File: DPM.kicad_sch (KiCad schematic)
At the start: 17 parts, among them J1 Conn_01x08, U1 74HC590, U2 74HC682, U3 ADG333A, U4 MCP23017_SP, U5 ADG333A

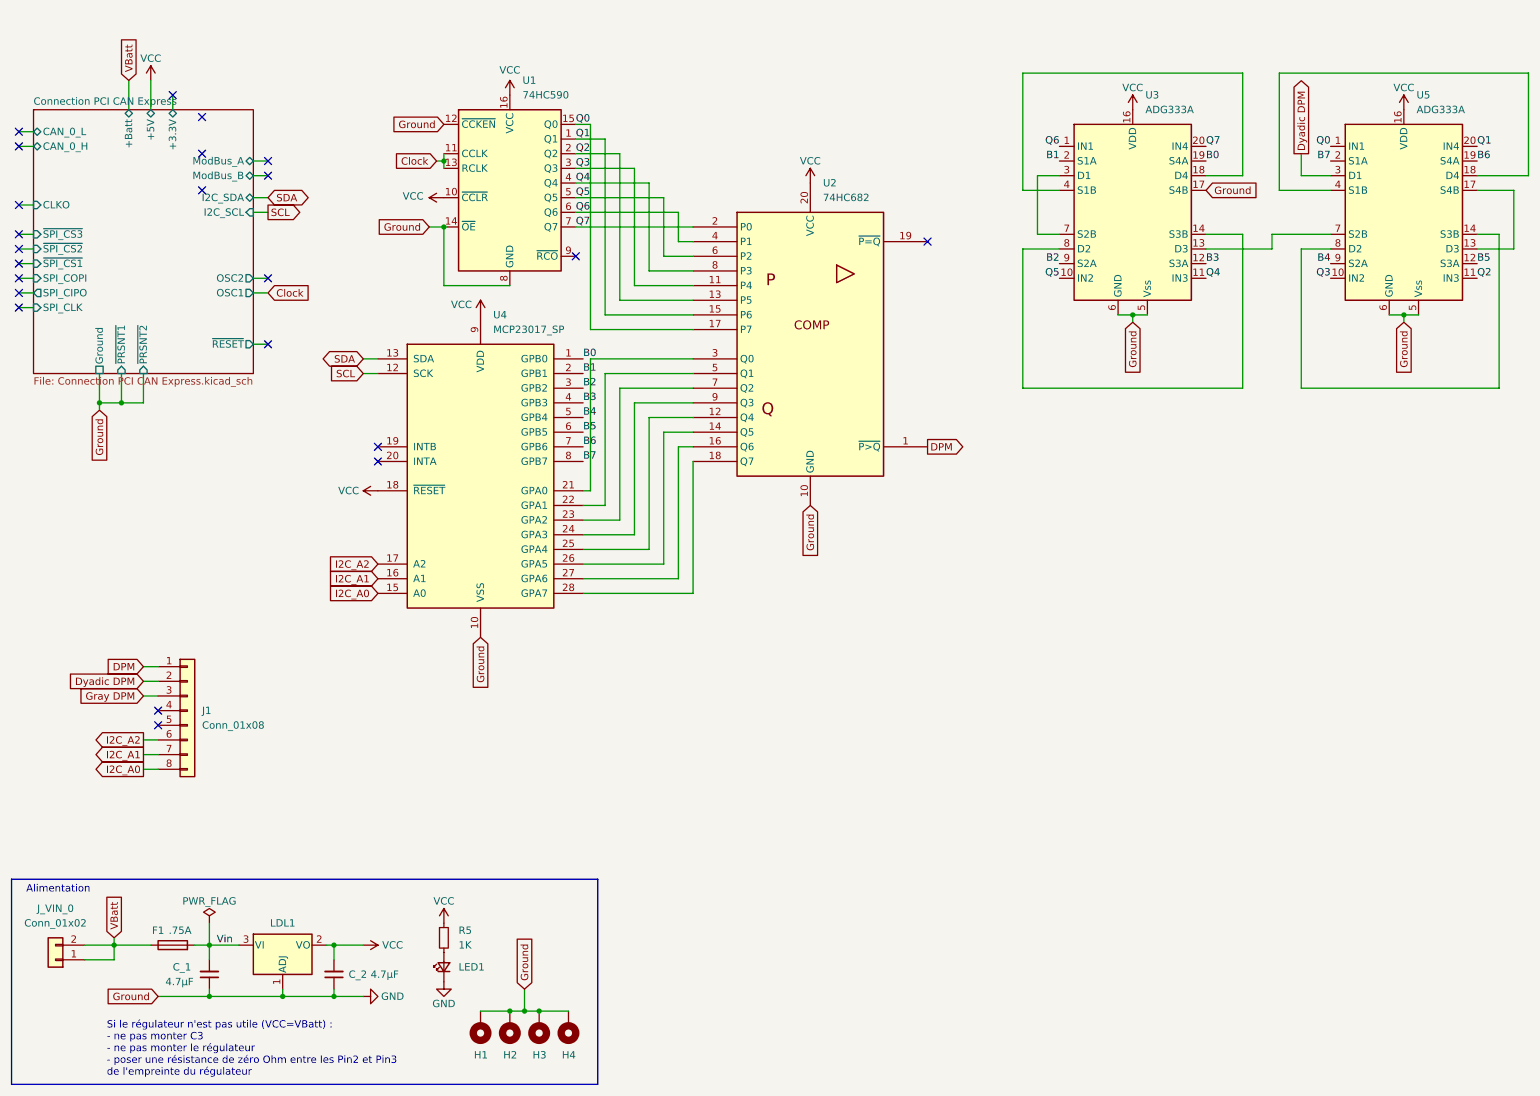
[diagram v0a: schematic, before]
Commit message: + 3 fonctionnalités : PWM, DPM & DDPM + début du routage de la carte
git-svn-id: file:///D%5C00%20-%20Dev%20&%20Calculs%5CRepoTortoiseSVN_PCB%5CD-DPM/trunk@16 f29d8339-a183-0348-962e-9e4594cf8312
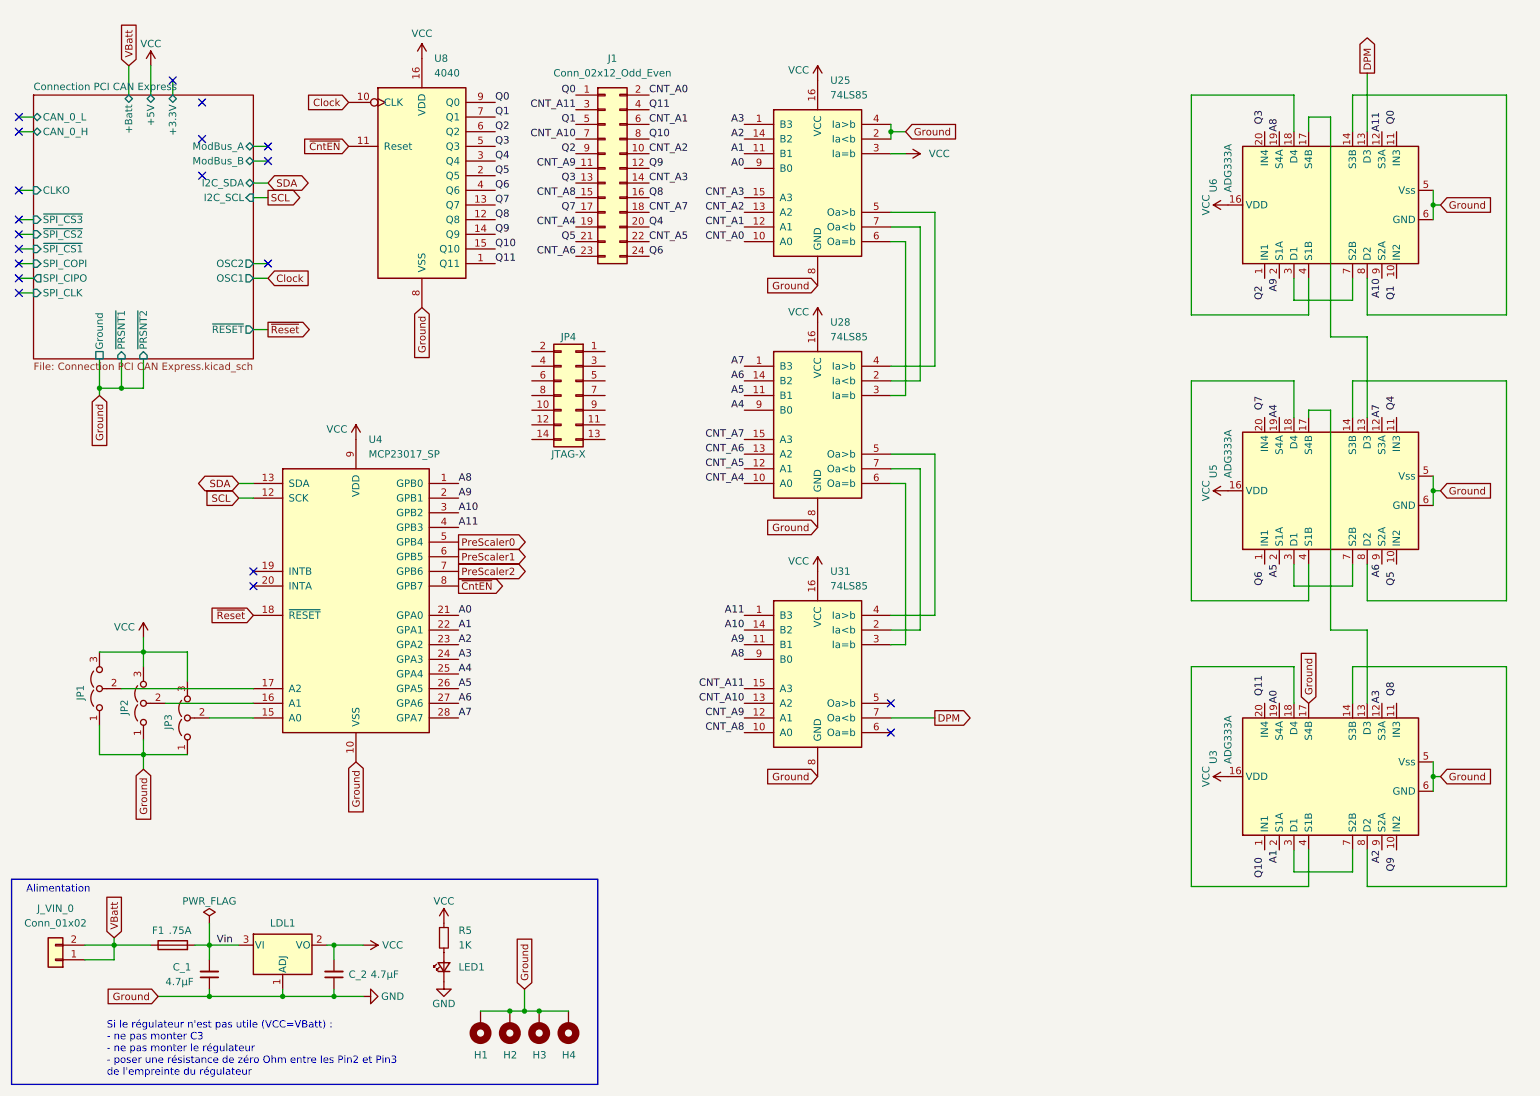
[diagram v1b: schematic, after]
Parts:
- removed J1: Conn_01x08, Connector_PinHeader_2.54mm:PinHeader_1x08_P2.54mm_Vertical, symbol Connector_Generic:Conn_01x08
- removed U1: 74HC590, Package_DIP:DIP-16_W7.62mm_Socket_LongPads, symbol Perso_Spare_parts:74HC590
- removed U2: 74HC682, Package_DIP:DIP-20_W7.62mm_Socket_LongPads, symbol Perso_Spare_parts:74HC682
- added J1: Conn_02x12_Odd_Even, Connector_PinHeader_2.54mm:PinHeader_2x12_P2.54mm_Vertical, symbol Connector_Generic:Conn_02x12_Odd_Even
- added JP1, JP2, JP3: Jumper_3_Open, Connector_PinHeader_2.54mm:PinHeader_1x03_P2.54mm_Vertical, symbol Jumper:Jumper_3_Open
- added JP4: JTAG-X, Connector_IDC:IDC-Header_2x07_P2.54mm_Horizontal, symbol Connector_Generic:Conn_02x07_Odd_Even
- added U25, U28, U31: 74LS85, Package_DIP:DIP-16_W7.62mm_Socket, symbol 74xx:74LS85
- added U6: ADG333A, Package_DIP:DIP-20_W7.62mm_Socket_LongPads, symbol Perso_Spare_parts:ADG333A
- added U8: 4040, Package_DIP:DIP-16_W7.62mm_Socket, symbol 4xxx:4040
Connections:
- net Clock: now also U8.10 (CLK)
- net DPM: now also U31.7 (Oa<b), U6.13 (D3)
- net GND: now also JP1.1 (A), JP2.1 (A), JP3.1 (A), U25.2 (Ia<b), U25.4 (Ia>b), U25.8 (GND), U28.8 (GND), U31.8 (GND), U6.15 (NC), U6.5 (Vss), U6.6 (GND), U8.8 (VSS)
- net Q0: now also J1.1 (Pin_1), U8.9 (Q0); no longer U5.1 (IN1)
- net Q1: now also J1.5 (Pin_5), U8.7 (Q1); no longer U5.20 (IN4)
- net Q2: now also J1.9 (Pin_9), U8.6 (Q2); no longer U5.11 (IN3)
- net Q3: now also J1.13 (Pin_13), U8.5 (Q3); no longer U5.10 (IN2)
- net Q4: now also J1.20 (Pin_20), U8.3 (Q4); no longer U3.11 (IN3)
- net Q5: now also J1.21 (Pin_21), U8.2 (Q5); no longer U3.10 (IN2)
- net Q6: now also J1.24 (Pin_24), U8.4 (Q6); no longer U3.1 (IN1)
- net Q7: now also J1.17 (Pin_17), U8.13 (Q7); no longer U3.20 (IN4)
- net VCC: now also JP1.3 (B), JP2.3 (B), JP3.3 (B), U25.16 (VCC), U25.3 (Ia=b), U28.16 (VCC), U31.16 (VCC), U6.16 (VDD), U8.16 (VDD); no longer U4.18 (~{RESET})
- net A0: now reaches U4.21 (GPA0)
- net A0: now also U3.19 (S4A), U25.9 (B0)
- net A1: now reaches U4.22 (GPA1)
- net A1: now also U3.2 (S1A), U25.11 (B1)
- net A2: now reaches U4.23 (GPA2)
- net A2: now also U3.9 (S2A), U25.14 (B2)
- net A3: now reaches U4.24 (GPA3)
- net A3: now also U3.12 (S3A), U25.1 (B3)
- net A4: now reaches U4.25 (GPA4)
- net A4: now also U5.19 (S4A), U28.9 (B0)
- net A5: now reaches U4.26 (GPA5)
- net A5: now also U5.2 (S1A), U28.11 (B1)
- net A6: now reaches U4.27 (GPA6)
- net A6: now also U5.9 (S2A), U28.14 (B2)
- net A7: now reaches U4.28 (GPA7)
- net A7: now also U5.12 (S3A), U28.1 (B3)
- net at U5.13 (D3): now also U6.17 (S4B); no longer U5.17 (S4B)
- net at U3.13 (D3): now also U5.17 (S4B); no longer U5.7 (S2B)
- net B0 renamed A8
- net A8: now also U31.9 (B0), U6.19 (S4A); no longer U3.19 (S4A)
- net B1 renamed A9
- net A9: now also U31.11 (B1), U6.2 (S1A); no longer U3.2 (S1A)
- net B2 renamed A10
- net A10: now also U31.14 (B2), U6.9 (S2A); no longer U3.9 (S2A)
- net B3 renamed A11
- net A11: now also U31.1 (B3), U6.12 (S3A); no longer U3.12 (S3A)
- net B4 renamed PreScaler0
- net PreScaler0: no longer U5.9 (S2A)
- net B5 renamed PreScaler1
- net PreScaler1: no longer U5.12 (S3A)
- net B6 renamed PreScaler2
- net PreScaler2: no longer U5.19 (S4A)
- net B7 renamed ~{CntEN}
- net ~{CntEN}: now also U8.11 (Reset); no longer U5.2 (S1A)
- net Dyadic DPM: no longer names the net of U5.3 (D1)
- net Dyadic DPM: now also U5.7 (S2B)
- net I2C_A0: no longer names the net of U4.15 (A0)
- net I2C_A0: now also JP3.2 (C)
- net I2C_A1: no longer names the net of U4.16 (A1)
- net I2C_A1: now also JP2.2 (C)
- net I2C_A2: no longer names the net of U4.17 (A2)
- net I2C_A2: now also JP1.2 (C)
- new net: U6.14 (S3B), U6.8 (D2)
- new net: U6.18 (D4), U6.4 (S1B)
- new net: U6.3 (D1), U6.7 (S2B)
- new net: U25.7 (Oa<b), U28.2 (Ia<b)
- new net: U25.6 (Oa=b), U28.3 (Ia=b)
- new net: U25.5 (Oa>b), U28.4 (Ia>b)
- new net: U28.5 (Oa>b), U31.4 (Ia>b)
- new net: U28.6 (Oa=b), U31.3 (Ia=b)
- new net: U28.7 (Oa<b), U31.2 (Ia<b)
- new net CNT_A0: J1.2 (Pin_2), U25.10 (A0)
- new net CNT_A1: J1.6 (Pin_6), U25.12 (A1)
- new net CNT_A10: J1.7 (Pin_7), U31.13 (A2)
- new net CNT_A11: J1.3 (Pin_3), U31.15 (A3)
- new net CNT_A2: J1.10 (Pin_10), U25.13 (A2)
- new net CNT_A3: J1.14 (Pin_14), U25.15 (A3)
- new net CNT_A4: J1.19 (Pin_19), U28.10 (A0)
- new net CNT_A5: J1.22 (Pin_22), U28.12 (A1)
- new net CNT_A6: J1.23 (Pin_23), U28.13 (A2)
- new net CNT_A7: J1.18 (Pin_18), U28.15 (A3)
- new net CNT_A8: J1.15 (Pin_15), U31.10 (A0)
- new net CNT_A9: J1.11 (Pin_11), U31.12 (A1)
- new net Q10: J1.8 (Pin_8), U8.15 (Q10)
- new net Q11: J1.4 (Pin_4), U8.1 (Q11)
- new net Q8: J1.16 (Pin_16), U8.12 (Q8)
- new net Q9: J1.12 (Pin_12), U8.14 (Q9)
- new net ~{Reset}: U4.18 (~{RESET})
- no-connect marks 23 -> 20
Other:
- moved on the sheet: U3, U4
